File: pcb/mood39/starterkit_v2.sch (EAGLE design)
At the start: 19 parts, among them IC1 TINY85, IC2 LP2950

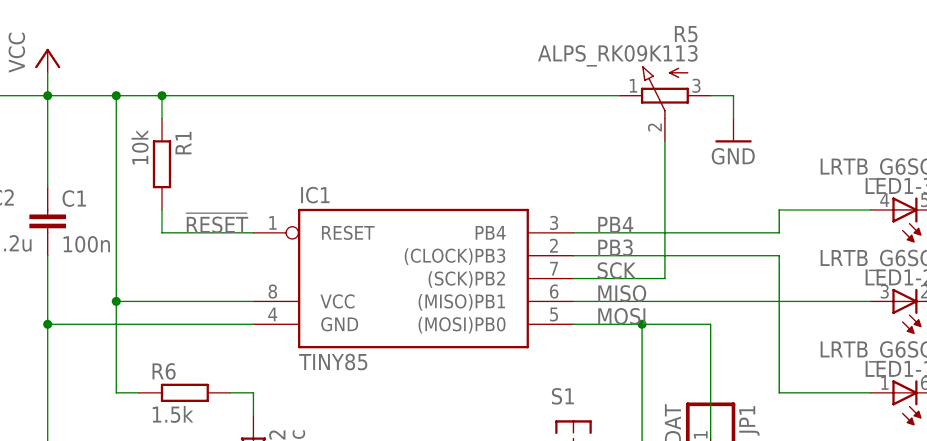
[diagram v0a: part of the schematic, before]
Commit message: routing almost done
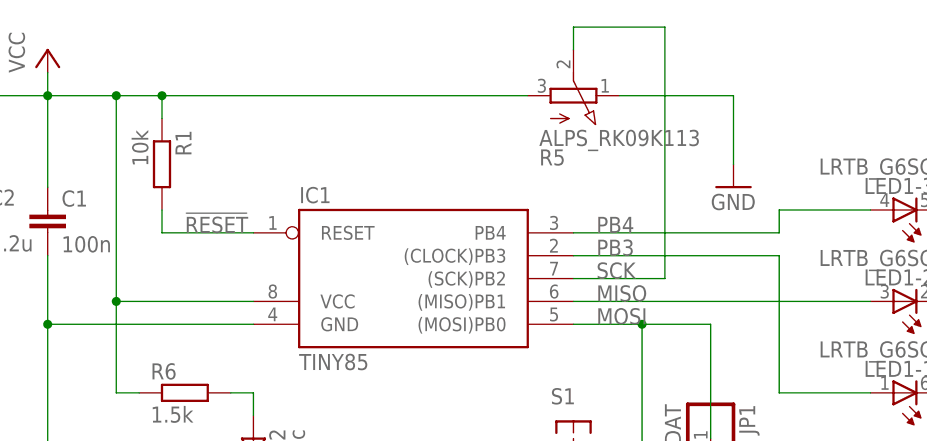
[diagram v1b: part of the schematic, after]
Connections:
- net GND: now also R5.E; no longer R5.A
- net VCC: now also R5.A; no longer R5.E
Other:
- moved on the sheet: R5
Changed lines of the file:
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@@
 <grid distance="0.1" unitdist="inch" unit="inch" style="lines" multiple="1" display="no" altdistance="0.01" altunitdist="inch" altunit="inch"/>
 <layers>
-<layer number="1" name="Top" color="4" fill="1" visible="yes" active="no"/>
-<layer number="16" name="Bottom" color="1" fill="1" visible="yes" active="no"/>
-<layer number="17" name="Pads" color="2" fill="1" visible="yes" active="no"/>
-<layer number="18" name="Vias" color="2" fill="1" visible="yes" active="no"/>
-<layer number="19" name="Unrouted" color="6" fill="1" visible="yes" active="no"/>
-<layer number="20" name="Dimension" color="15" fill="1" visible="yes" active="no"/>
-<layer number="21" name="tPlace" color="7" fill="1" visible="yes" active="no"/>
-<layer number="22" name="bPlace" color="7" fill="1" visible="yes" active="no"/>
-<layer number="23" name="tOrigins" color="15" fill="1" visible="yes" active="no"/>
-<layer number="24" name="bOrigins" color="15" fill="1" visible="yes" active="no"/>
-<layer number="25" name="tNames" color="7" fill="1" visible="yes" active="no"/>
-<layer number="26" name="bNames" color="7" fill="1" visible="yes" active="no"/>
-<layer number="27" name="tValues" color="7" fill="1" visible="yes" active="no"/>
-<layer number="28" name="bValues" color="7" fill="1" visible="yes" active="no"/>
+<layer number="1" name="Top" color="4" fill="1" visible="no" active="no"/>
+<layer number="16" name="Bottom" color="1" fill="1" visible="no" active="no"/>
+<layer number="17" name="Pads" color="2" fill="1" visible="no" active="no"/>
+<layer number="18" name="Vias" color="2" fill="1" visible="no" active="no"/>
+<layer number="19" name="Unrouted" color="6" fill="1" visible="no" active="no"/>
+<layer number="20" name="Dimension" color="15" fill="1" visible="no" active="no"/>
+<layer number="21" name="tPlace" color="7" fill="1" visible="no" active="no"/>
+<layer number="22" name="bPlace" color="7" fill="1" visible="no" active="no"/>
+<layer number="23" name="tOrigins" color="15" fill="1" visible="no" active="no"/>
+<layer number="24" name="bOrigins" color="15" fill="1" visible="no" active="no"/>
+<layer number="25" name="tNames" color="7" fill="1" visible="no" active="no"/>
+<layer number="26" name="bNames" color="7" fill="1" visible="no" active="no"/>
+<layer number="27" name="tValues" color="7" fill="1" visible="no" active="no"/>
+<layer number="28" name="bValues" color="7" fill="1" visible="no" active="no"/>
 <layer number="29" name="tStop" color="7" fill="3" visible="no" active="no"/>
 <layer number="30" name="bStop" color="7" fill="6" visible="no" active="no"/>
@@
 <layer number="35" name="tGlue" color="7" fill="4" visible="no" active="no"/>
 <layer number="36" name="bGlue" color="7" fill="5" visible="no" active="no"/>
-<layer number="37" name="tTest" color="7" fill="1" visible="yes" active="no"/>
-<layer number="38" name="bTest" color="7" fill="1" visible="yes" active="no"/>
+<layer number="37" name="tTest" color="7" fill="1" visible="no" active="no"/>
+<layer number="38" name="bTest" color="7" fill="1" visible="no" active="no"/>
 <layer number="39" name="tKeepout" color="4" fill="11" visible="no" active="no"/>
 <layer number="40" name="bKeepout" color="1" fill="11" visible="no" active="no"/>
@@
 <layer number="44" name="Drills" color="7" fill="1" visible="no" active="no"/>
 <layer number="45" name="Holes" color="7" fill="1" visible="no" active="no"/>
-<layer number="46" name="Milling" color="3" fill="1" visible="yes" active="no"/>
-<layer number="47" name="Measures" color="7" fill="1" visible="yes" active="no"/>
-<layer number="48" name="Document" color="7" fill="1" visible="yes" active="no"/>
-<layer number="49" name="Reference" color="7" fill="1" visible="yes" active="no"/>
-<layer number="51" name="tDocu" color="7" fill="1" visible="yes" active="no"/>
-<layer number="52" name="bDocu" color="7" fill="1" visible="yes" active="no"/>
+<layer number="46" name="Milling" color="3" fill="1" visible="no" active="no"/>
+<layer number="47" name="Measures" color="7" fill="1" visible="no" active="no"/>
+<layer number="48" name="Document" color="7" fill="1" visible="no" active="no"/>
+<layer number="49" name="Reference" color="7" fill="1" visible="no" active="no"/>
+<layer number="51" name="tDocu" color="7" fill="1" visible="no" active="no"/>
+<layer number="52" name="bDocu" color="7" fill="1" visible="no" active="no"/>
 <layer number="91" name="Nets" color="2" fill="1" visible="yes" active="yes"/>
 <layer number="92" name="Busses" color="1" fill="1" visible="yes" active="yes"/>
@@
 <instance part="IC2" gate="G$1" x="-5.08" y="91.44"/>
 <instance part="C2" gate="G$1" x="7.62" y="78.74"/>
-<instance part="R5" gate="R$1" x="83.82" y="91.44" rot="MR270"/>
+<instance part="R5" gate="R$1" x="73.66" y="91.44" rot="MR90"/>
 <instance part="JP1" gate="G$1" x="88.9" y="50.8" rot="R270"/>
-<instance part="GND2" gate="1" x="91.44" y="86.36"/>
+<instance part="GND2" gate="1" x="91.44" y="81.28"/>
 <instance part="LED2" gate="G$1" x="38.1" y="53.34"/>
 <instance part="R6" gate="G$1" x="30.48" y="58.42"/>
@@
 </segment>
 <segment>
-<pinref part="R5" gate="R$1" pin="A"/>
-<wire x1="88.9" y1="91.44" x2="91.44" y2="91.44" width="0.1524" layer="91"/>
-<wire x1="91.44" y1="91.44" x2="91.44" y2="88.9" width="0.1524" layer="91"/>
 <pinref part="GND2" gate="1" pin="GND"/>
+<wire x1="91.44" y1="83.82" x2="91.44" y2="91.44" width="0.1524" layer="91"/>
+<pinref part="R5" gate="R$1" pin="E"/>
+<wire x1="91.44" y1="91.44" x2="78.74" y2="91.44" width="0.1524" layer="91"/>
 </segment>
 </net>
@@
 <wire x1="7.62" y1="81.28" x2="7.62" y2="91.44" width="0.1524" layer="91"/>
 <junction x="7.62" y="91.44"/>
-<pinref part="R5" gate="R$1" pin="E"/>
 <wire x1="22.86" y1="91.44" x2="27.94" y2="91.44" width="0.1524" layer="91"/>
 <pinref part="R1" gate="G$1" pin="1"/>
-<wire x1="27.94" y1="91.44" x2="78.74" y2="91.44" width="0.1524" layer="91"/>
 <wire x1="27.94" y1="88.9" x2="27.94" y2="91.44" width="0.1524" layer="91"/>
-<junction x="27.94" y="91.44"/>
 <wire x1="22.86" y1="68.58" x2="22.86" y2="58.42" width="0.1524" layer="91"/>
 <pinref part="R6" gate="G$1" pin="1"/>
 <wire x1="22.86" y1="58.42" x2="25.4" y2="58.42" width="0.1524" layer="91"/>
 <junction x="22.86" y="68.58"/>
+<pinref part="R5" gate="R$1" pin="A"/>
+<wire x1="68.58" y1="91.44" x2="27.94" y2="91.44" width="0.1524" layer="91"/>
+<junction x="27.94" y="91.44"/>
 </segment>
 <segment>
@@
 <label x="76.2" y="71.12" size="1.778" layer="95"/>
 <pinref part="R5" gate="R$1" pin="S"/>
-<wire x1="83.82" y1="86.36" x2="83.82" y2="71.12" width="0.1524" layer="91"/>
-</segment>
-<segment>
+<wire x1="73.66" y1="96.52" x2="73.66" y2="99.06" width="0.1524" layer="91"/>
+<wire x1="73.66" y1="99.06" x2="83.82" y2="99.06" width="0.1524" layer="91"/>
+<wire x1="83.82" y1="99.06" x2="83.82" y2="71.12" width="0.1524" layer="91"/>
+</segment>
+<segment>
